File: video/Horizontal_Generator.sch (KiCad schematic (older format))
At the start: 10 parts, among them U10 74LS08, U11 74LS08, U15 74LS08, U16 74LS04, U17 74LS02, U18 74LS08, U19 74LS163, U2 74LS02, U20 74LS163, U21 74LS163

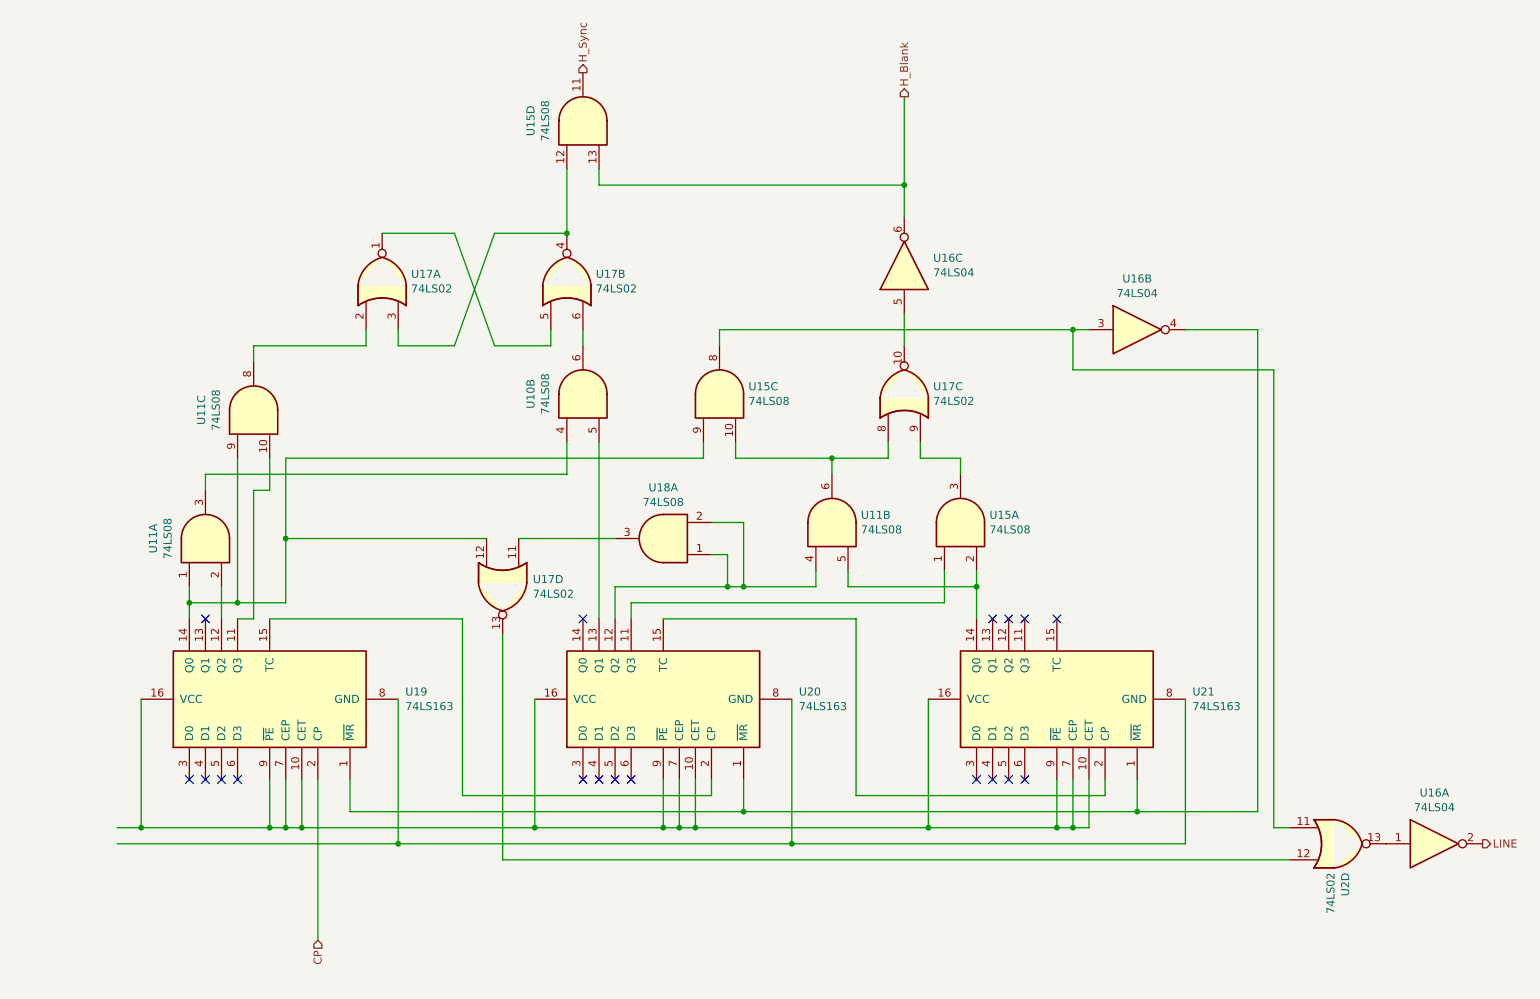
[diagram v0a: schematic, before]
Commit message: Resize and plot video
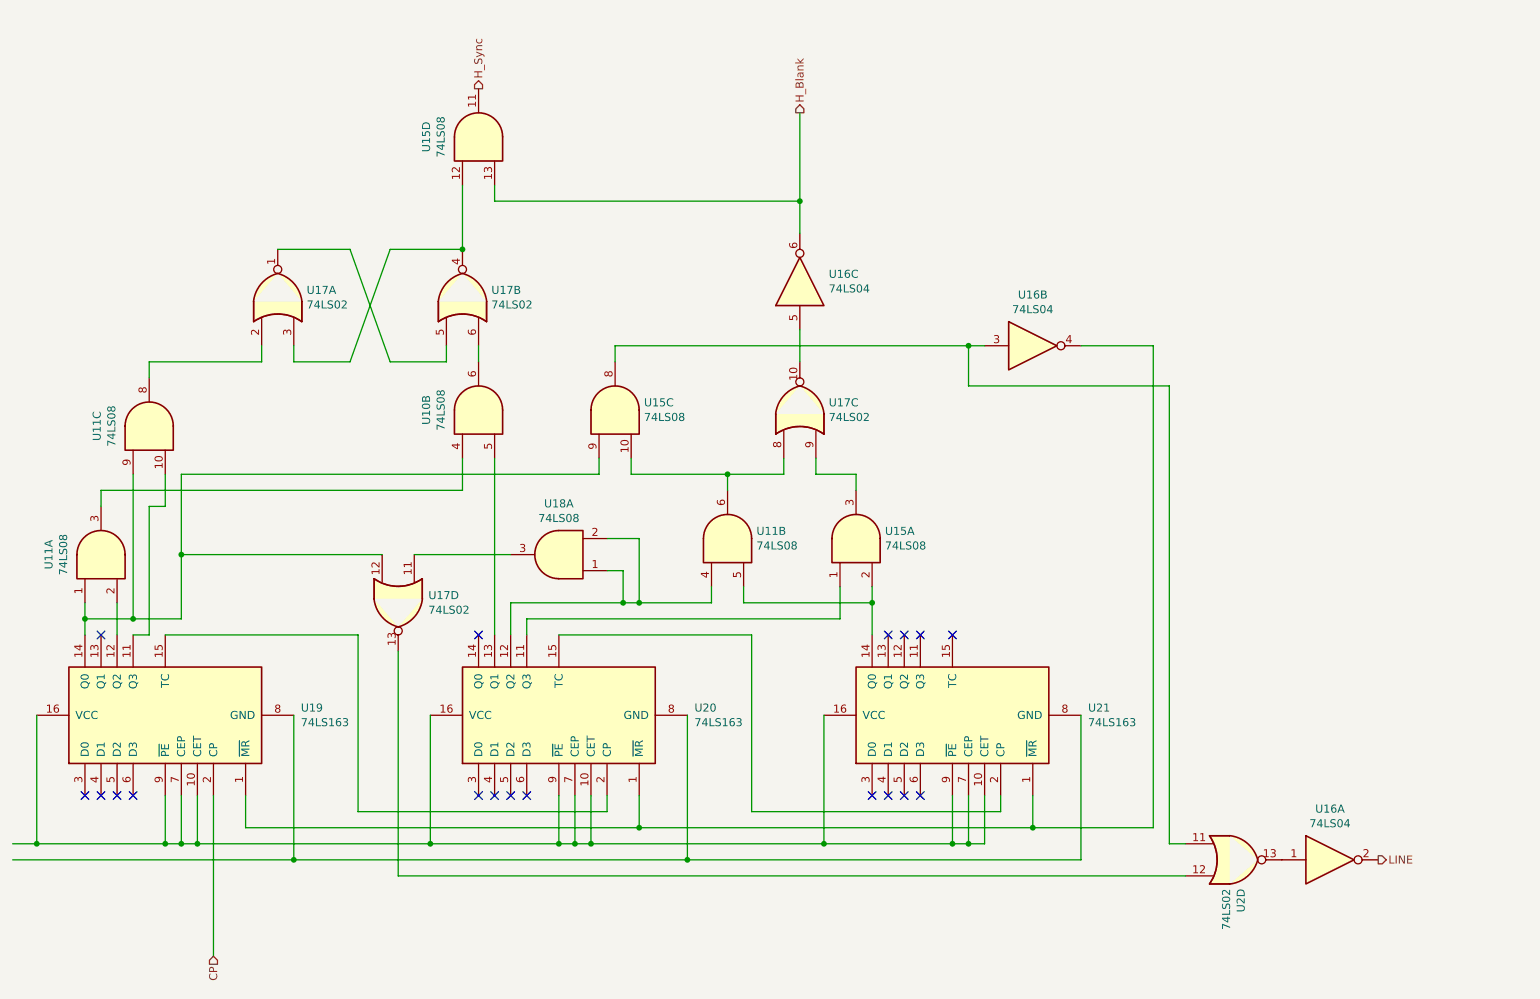
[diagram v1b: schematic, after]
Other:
- moved on the sheet: U10B, U11A, U11B, U11C, U15A, U15C, U15D, U16A, U16B, U16C, U17A, U17B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
